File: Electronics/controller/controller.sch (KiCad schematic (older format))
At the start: 26 parts, among them P1 POWER, P2 PANEL_1, P3 PANEL_2, Q1 P55NF, SW1 SW_PUSH, U1 LM7805CT, U2 74HC595, U3 Arduino_Pro_Micro

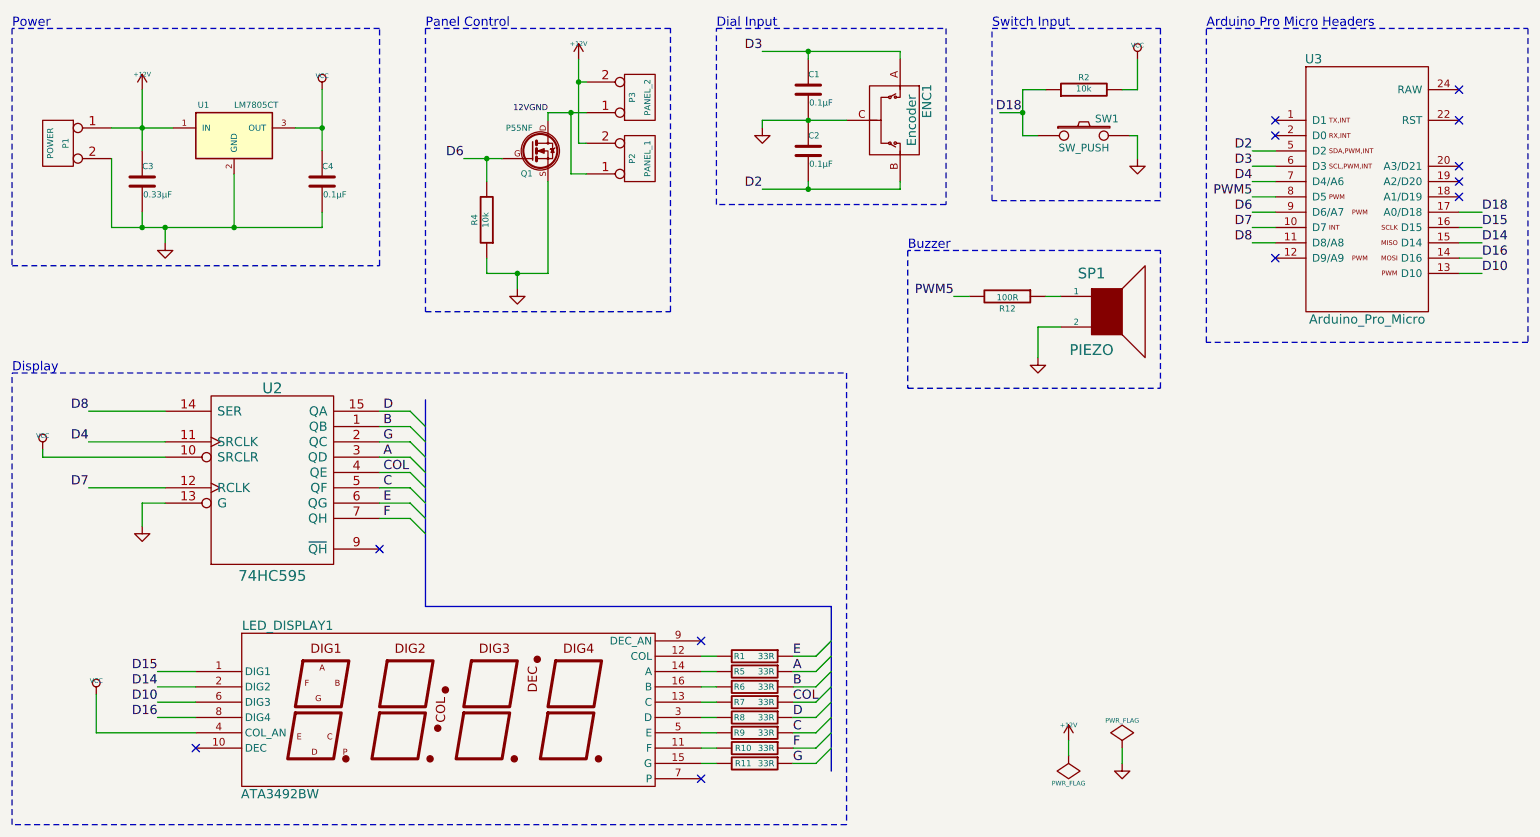
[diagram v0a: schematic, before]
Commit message: Moved some parts around on the board.
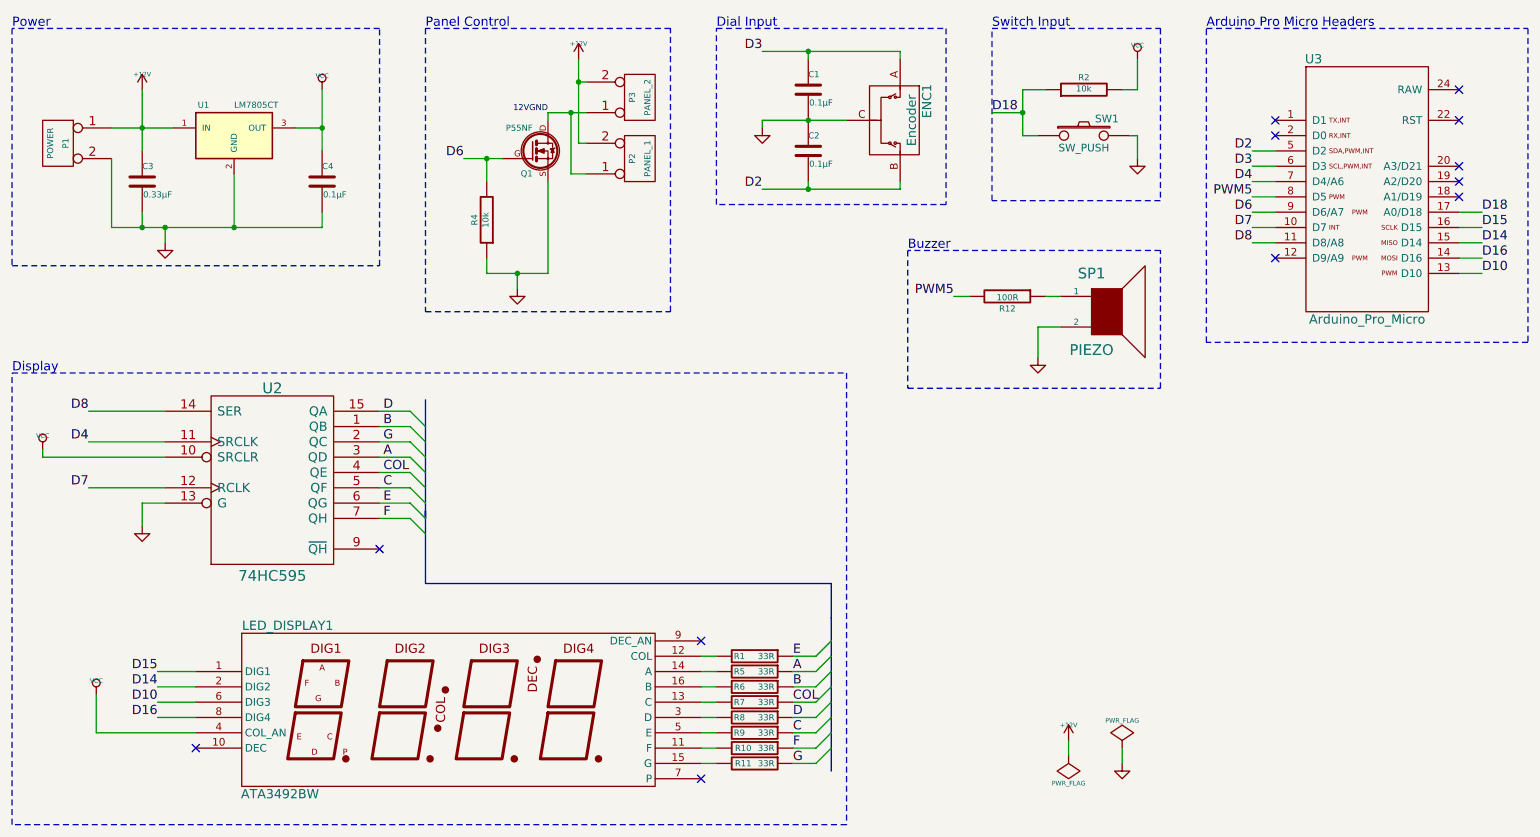
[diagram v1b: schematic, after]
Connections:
- net D18: now also R2.1, SW1.1
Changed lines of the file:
@@
 EESchema Schematic File Version 2
-LIBS:cylindric
-LIBS:borniers
 LIBS:power
 LIBS:device
@@
 LIBS:contrib
 LIBS:valves
-LIBS:controller-cache
+LIBS:borniers
+LIBS:cylindric
+LIBS:digit_board-cache
 EELAYER 25 0
 EELAYER END
@@
 	1    0    0    -1
 $EndComp
-Text Label 7225 1300 0    60   ~ 0
+Text Label 7200 1300 0    60   ~ 0
 D18
 Text Notes 7200 750  0    60   ~ 0
@@
 	4100 2350 4100 2450
 Wire Wire Line
-	3900 2350 4300 2350
+	3900 2350 4100 2350
+Wire Wire Line
+	4100 2350 4300 2350
 Wire Wire Line
 	4500 1500 4550 1500
@@
 	4450 1700 4550 1700
 Wire Wire Line
-	4500 950  4500 1500
+	4500 950  4500 1100
+Wire Wire Line
+	4500 1100 4500 1500
 Wire Wire Line
 	4500 1100 4550 1100
@@
 	3900 2250 3900 2350
 Wire Wire Line
-	5700 1800 6600 1800
-Wire Wire Line
-	5700 1350 6250 1350
-Wire Wire Line
-	1450 1400 1850 1400
+	5700 1800 6000 1800
+Wire Wire Line
+	6000 1800 6600 1800
+Wire Wire Line
+	5700 1350 6000 1350
+Wire Wire Line
+	6000 1350 6250 1350
+Wire Wire Line
+	1450 1400 1650 1400
+Wire Wire Line
+	1650 1400 1850 1400
 Connection ~ 1650 1400
 Wire Wire Line
-	1650 1150 1650 1550
+	1650 1150 1650 1400
+Wire Wire Line
+	1650 1400 1650 1550
 Wire Wire Line
 	2250 2050 2250 1700
 Wire Wire Line
-	1450 2050 2825 2050
+	1450 2050 1650 2050
+Wire Wire Line
+	1650 2050 1800 2050
+Wire Wire Line
+	1800 2050 2250 2050
+Wire Wire Line
+	2250 2050 2825 2050
 Connection ~ 1800 2050
 Wire Notes Line
@@
 	10700 2800 8600 2800
 Wire Wire Line
-	5700 900  6600 900
+	5700 900  6000 900
+Wire Wire Line
+	6000 900  6600 900
 Wire Wire Line
 	5700 1350 5700 1400
@@
 	4300 1350 4300 1300
 Wire Wire Line
-	4300 1300 4550 1300
+	4300 1300 4450 1300
+Wire Wire Line
+	4450 1300 4550 1300
 Wire Wire Line
 	3900 1750 3900 1600
 Wire Wire Line
-	3750 1600 4000 1600
+	3750 1600 3900 1600
+Wire Wire Line
+	3900 1600 4000 1600
 Wire Wire Line
 	3200 3250 3400 3250
@@
 	1350 5350 1350 5100
 Wire Bus Line
-	3500 4525 6150 4525
+	3500 4375 6150 4375
 Entry Wire Line
 	3400 3250 3500 3350
@@
 	3400 3950 3500 4050
 Wire Bus Line
-	3500 3175 3500 4525
+	3500 3175 3500 3350
+Wire Bus Line
+	3500 3350 3500 3450
+Wire Bus Line
+	3500 3450 3500 3550
+Wire Bus Line
+	3500 3550 3500 3650
+Wire Bus Line
+	3500 3650 3500 3750
+Wire Bus Line
+	3500 3750 3500 3850
+Wire Bus Line
+	3500 3850 3500 3950
+Wire Bus Line
+	3500 3950 3500 3900
+Wire Bus Line
+	3500 3900 3500 4375
 Entry Wire Line
 	6050 4850 6150 4750
@@
 	6050 5550 6150 5450
 Wire Bus Line
-	6150 4525 6150 5600
+	6150 4375 6150 4600
+Wire Bus Line
+	6150 4600 6150 4750
+Wire Bus Line
+	6150 4750 6150 4850
+Wire Bus Line
+	6150 4850 6150 4950
+Wire Bus Line
+	6150 4950 6150 5050
+Wire Bus Line
+	6150 5050 6150 5150
+Wire Bus Line
+	6150 5150 6150 5250
+Wire Bus Line
+	6150 5250 6150 5350
+Wire Bus Line
+	6150 5350 6150 5450
+Wire Bus Line
+	6150 5450 6150 5600
 Wire Wire Line
 	9050 2050 8900 2050
@@
 $EndComp
 Wire Wire Line
-	2825 1150 2825 1550
+	2825 1150 2825 1400
+Wire Wire Line
+	2825 1400 2825 1550
 Connection ~ 2825 1400
 Wire Wire Line
@@
 $EndComp
 Wire Wire Line
-	7400 1150 7400 1450
+	7400 1150 7400 1300
+Wire Wire Line
+	7400 1300 7400 1450
 Wire Wire Line
 	7400 1450 7500 1450
@@
 $EndComp
 Wire Wire Line
-	7400 1300 7250 1300
+	7400 1300 7200 1300
 Connection ~ 7400 1300
 $EndSCHEMATC
